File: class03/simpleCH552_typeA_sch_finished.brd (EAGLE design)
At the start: 40.6 x 12 mm, 15 parts, among them U2 CH552G, X1 USBPCB

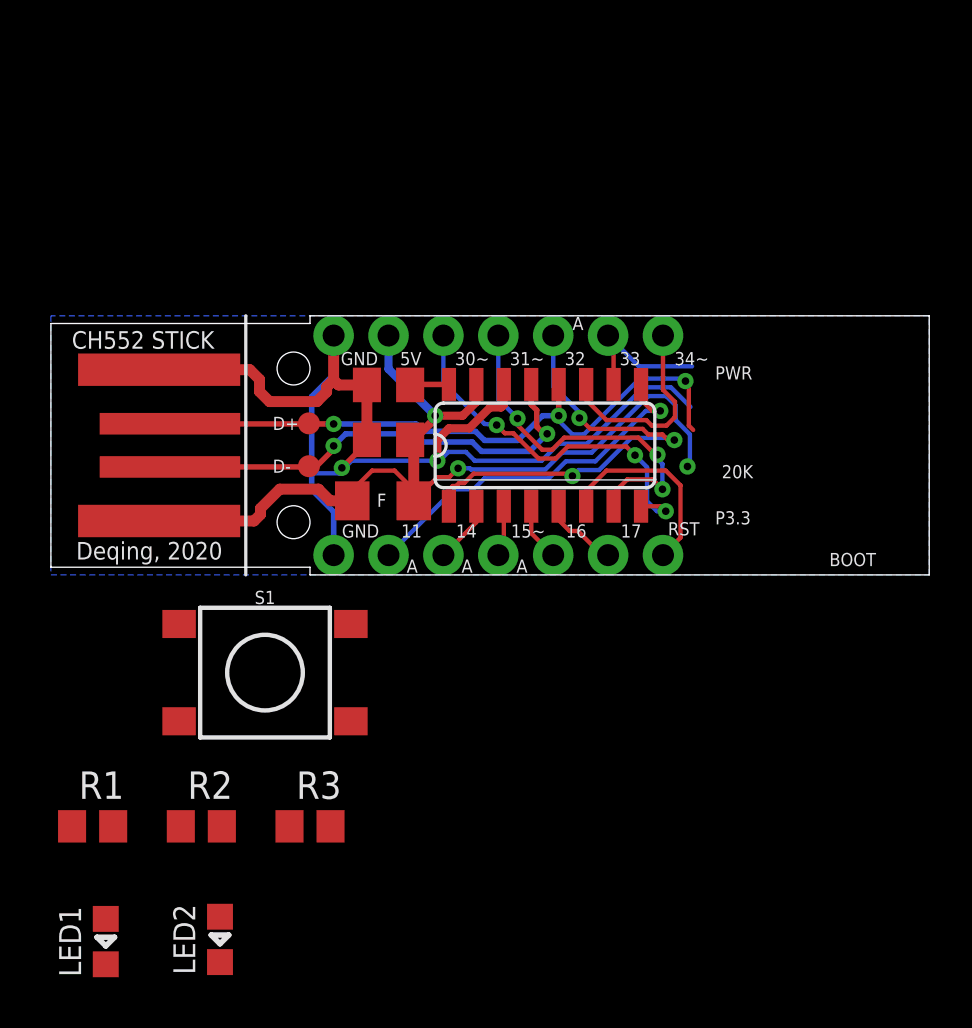
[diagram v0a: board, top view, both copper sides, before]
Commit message: change sch finished
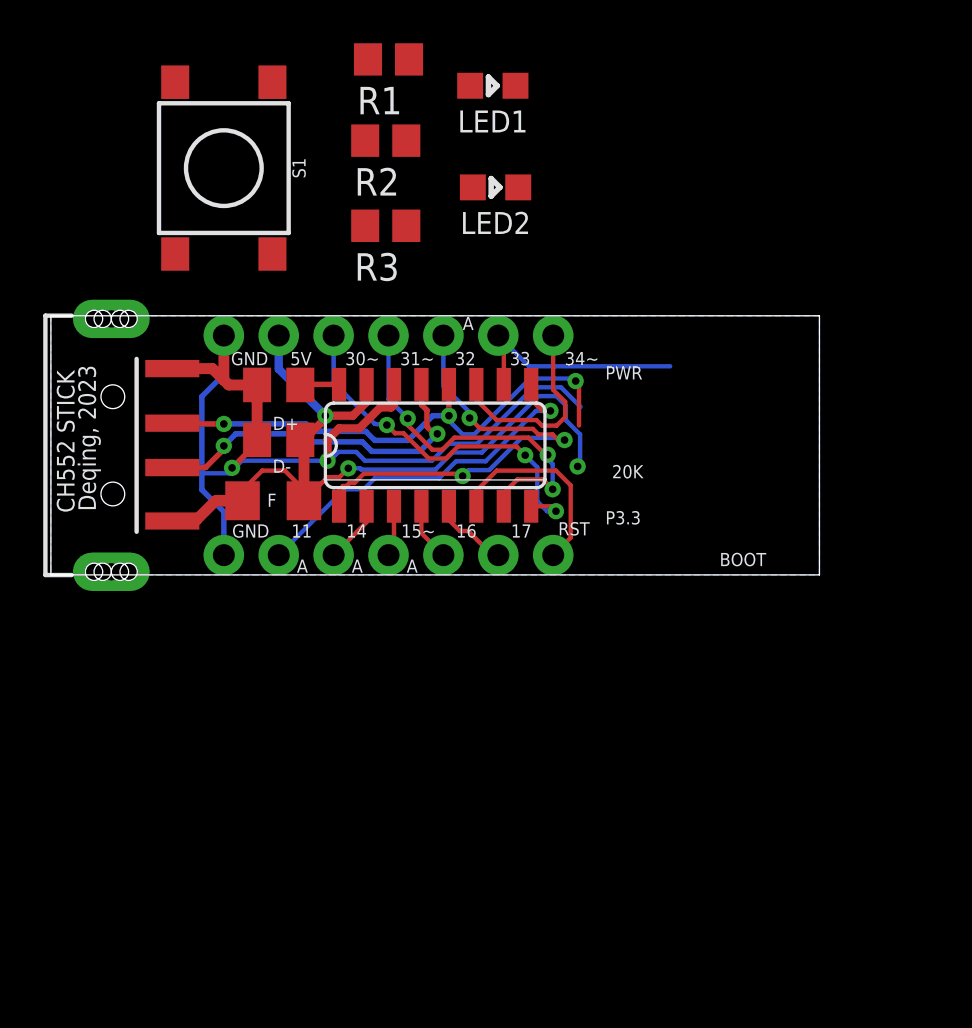
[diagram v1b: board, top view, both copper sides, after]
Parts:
- removed TP1, TP2: TEST-POINT3X4, SparkFun-Connectors:PAD.03X.04
- removed X1: USBPCB, SparkFun:USB-A-PCB
- added J4: USB_A_SMT_MALE, SparkFun-Connectors:USB-A-SMT-MALE
- moved LED1 43.5 mm to (20.4, 22.6), turned to 90 degrees
- moved R1 38.0 mm to (15.6, 23.9), turned to 180 degrees
- moved LED2 37.1 mm to (20.6, 17.9), turned to 90 degrees
- moved R2 32.9 mm to (15.5, 20.1), turned to 180 degrees
- moved R3 28.0 mm to (15.5, 16.2), turned to 180 degrees
- moved S1 23.4 mm to (8.00, 18.8), turned to 270 degrees
- moved C1 5.08 mm to (10.5, 6.25)
- moved C2 5.08 mm to (10.5, 8.79)
- moved F1 5.08 mm to (10.3, 3.43)
- moved J1 5.08 mm to (8.00, 0.91)
- moved J2 5.08 mm to (8.00, 11.1)
- moved U2 5.08 mm to (17.8, 5.99)
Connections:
- net +5V: now also J4.VBUS1; no longer X1.5V
- net GND: now also J4.GND1; no longer X1.GND
- net USB_D+: now also J4.D+1; no longer TP2.P$1, X1.USB_P
- net USB_D-: now also J4.D-1; no longer TP1.P$1, X1.USB_M
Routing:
- net GND: track 54.1 -> 47.2 mm
- net USB_D+: track 31.3 -> 24.7 mm
- net USB_D-: track 21.9 -> 16.4 mm
- net +5V: track 43.8 -> 38.7 mm
- net P3.3: track 6.84 -> 10.9 mm
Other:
- board size 40.6 x 12 mm -> 35.6 x 12 mm
- board text added: "Deqing Sun 2023"
- board text added: "Deqing Sun, 2023 Prototyping Electronic Devices"
- board text added: "Deqing, 2023"
- board text added: "Try Ch55xduino with this board"
- board text removed: "Deqing Sun, 2020 Try Ch55xduino with this board"
- board text removed: "Deqing Sun, 2022 Prototyping Electronic Devices"
- board text removed: "Deqing, 2020"
